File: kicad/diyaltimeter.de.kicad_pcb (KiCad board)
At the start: 2 copper layers, 45.7 x 73.7 mm, 8 parts, among them J1 Buttons, J2 Display, J3 links, J4 rechts, J5 I2C_BMP280, J6 I2C_BMP280_2, J7 RTC DS3231

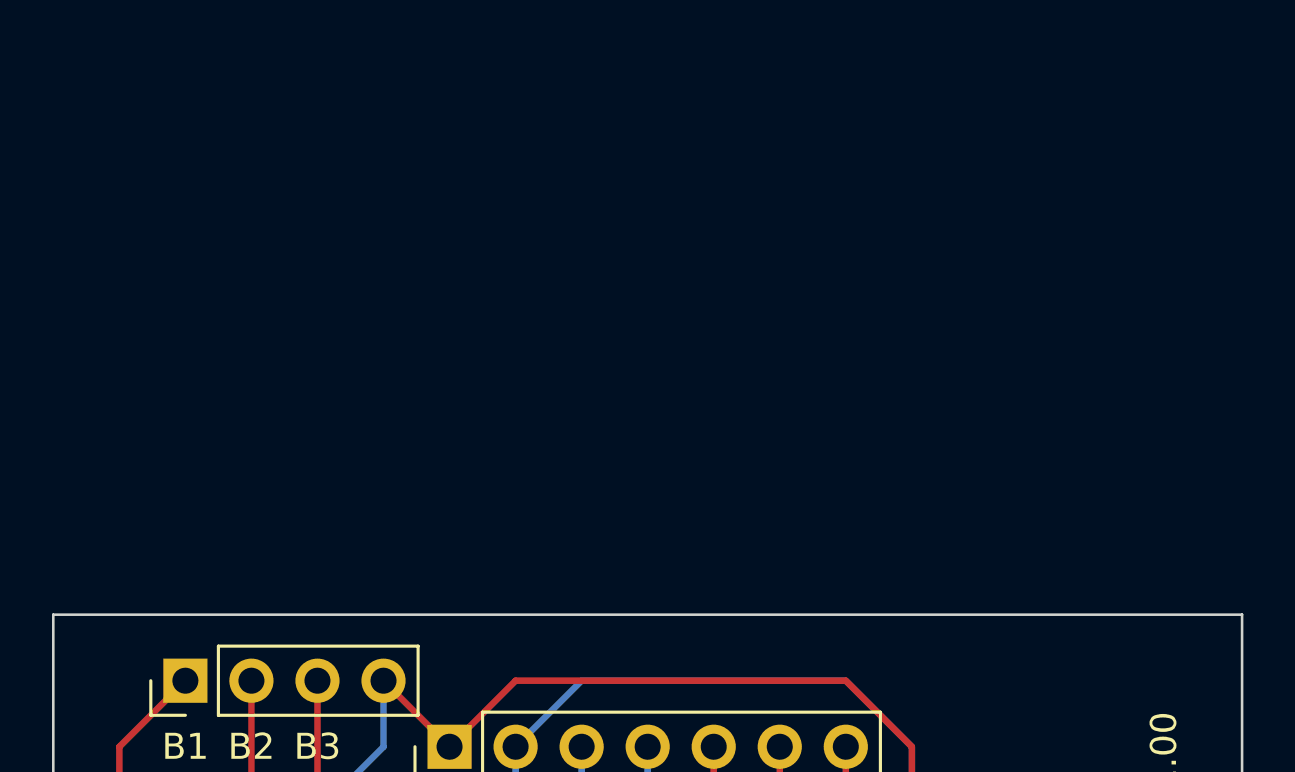
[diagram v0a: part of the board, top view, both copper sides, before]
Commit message: updated pcb
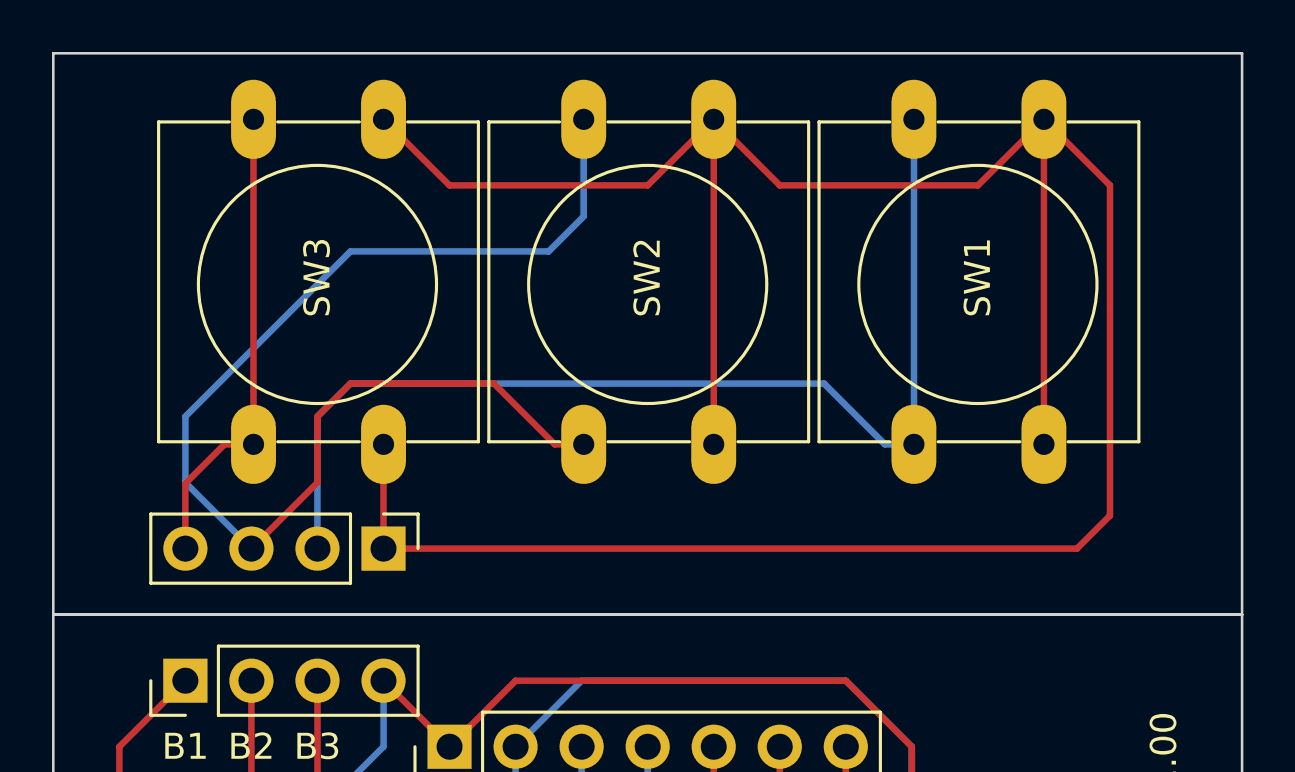
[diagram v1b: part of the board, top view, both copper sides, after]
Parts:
- added J8: Conn_01x04_Male, Connector_PinHeader_2.54mm:PinHeader_1x04_P2.54mm_Vertical, F.Cu at (78.7, 104.1)
- added SW1: SW_Push, Button_Switch_THT:SW_PUSH-12mm, F.Cu at (104.1, 87.6)
- added SW2: SW_Push, Button_Switch_THT:SW_PUSH-12mm, F.Cu at (91.4, 87.6)
- added SW3: SW_Push, Button_Switch_THT:SW_PUSH-12mm, F.Cu at (78.7, 87.6)
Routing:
- net Net-(J8-Pad1): track 0.00 -> 103.4 mm
- net Net-(J8-Pad3): track 0.00 -> 46.2 mm
- net Net-(J8-Pad2): track 0.00 -> 42.7 mm
- net Net-(J8-Pad4): track 0.00 -> 18.2 mm
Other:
- board size 45.7 x 73.7 mm -> 45.7 x 95.2 mm
- net class Default: trace_width 0.25 -> 0.4
- rule trace_min: 0.2 -> 0.4

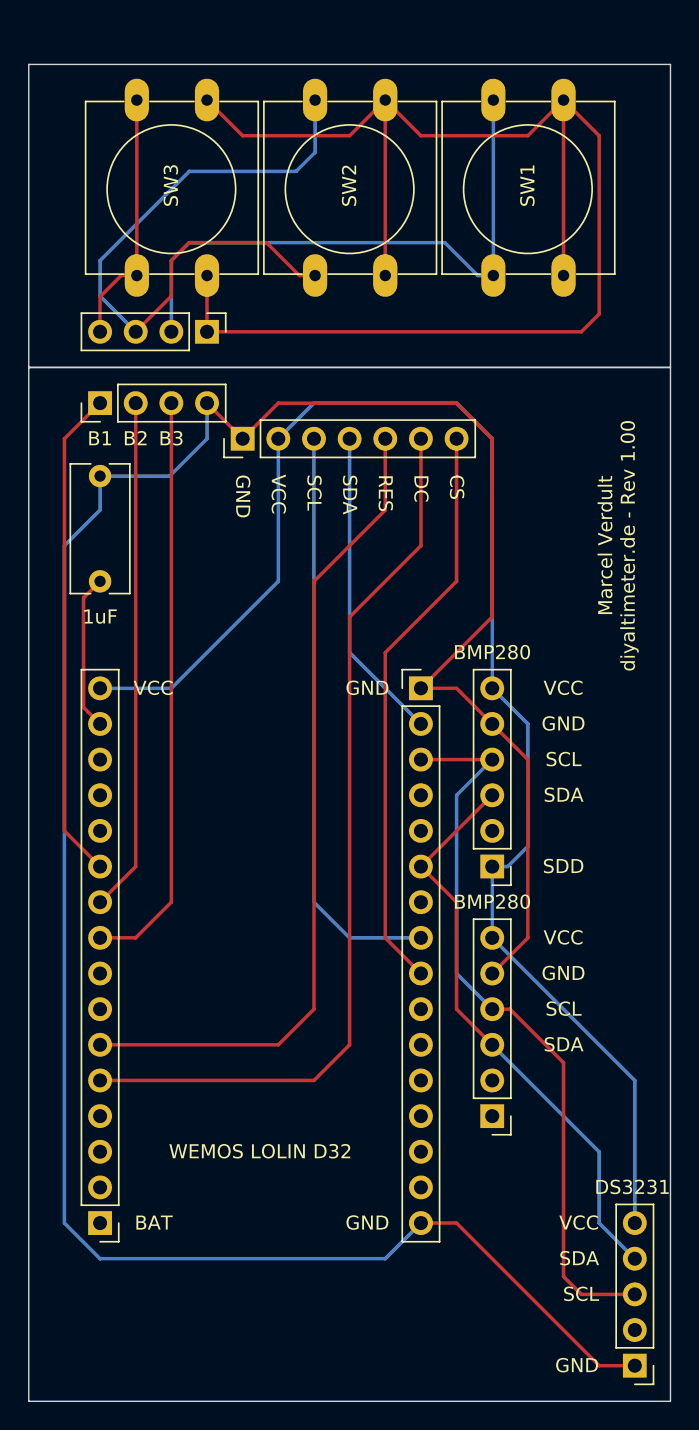
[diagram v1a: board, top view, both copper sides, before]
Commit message: pcb v1.01
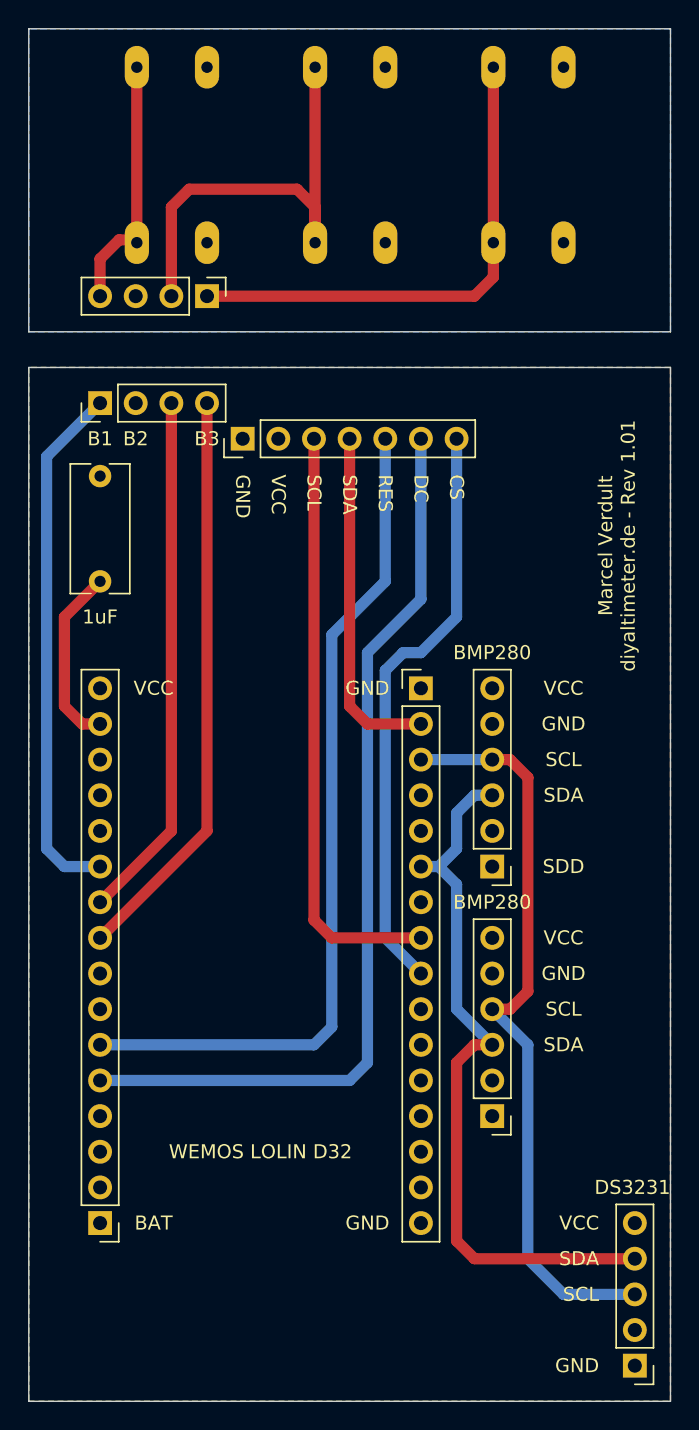
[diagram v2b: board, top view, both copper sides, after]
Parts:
- SW1, SW2, SW3: moved to B.Cu
- moved SW1 10.2 mm to (104.1, 97.8), turned to 90 degrees
- moved SW2 10.2 mm to (91.4, 97.8), turned to 90 degrees
- moved SW3 10.2 mm to (78.7, 97.8), turned to 90 degrees
- moved J8 2.54 mm to (78.7, 101.6)
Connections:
- J1 pad 2: 33 -> GND
- J1 pad 3: 25 -> 33
- J1 pad 4: GND -> 25
- SW1 pad 1: Net-(J8-Pad1) -> Net-(J8-Pad3)
- SW1 pad 2: Net-(J8-Pad2) -> Net-(J8-Pad1)
- SW2 pad 1: Net-(J8-Pad1) -> Net-(J8-Pad3)
- SW2 pad 2: Net-(J8-Pad3) -> Net-(J8-Pad2)
- SW3 pad 1: Net-(J8-Pad1) -> Net-(J8-Pad3)
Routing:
- net GND: track 181.9 -> 0.00 mm
- net +3V3: track 106.2 -> 0.00 mm, vias 0 -> 1
- net Net-(J8-Pad1): track 103.4 -> 36.1 mm
- net Net-(J8-Pad3): track 46.2 -> 0.00 mm
- net I2C_SDA: track 41.4 -> 51.9 mm
- net Net-(J8-Pad2): track 42.7 -> 33.6 mm
- net 32: track 35.1 -> 37.7 mm
- net SDA: track 22.4 -> 24.7 mm
- net RS: track 11.1 -> 13.0 mm
- net DC: track 64.1 -> 65.6 mm
- net RES: track 59.0 -> 60.5 mm
- net I2C_SCL: track 52.5 -> 54.0 mm
- net 33: track 36.6 -> 37.7 mm
- net SCL: track 41.7 -> 42.4 mm
- net CS: track 41.3 -> 42.0 mm
- added copper zone on B.Cu, net +3V3
- added copper zone on F.Cu, net GND
- added copper zone on B.Cu, net Net-(J8-Pad3)
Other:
- board size 45.7 x 95.2 mm -> 45.7 x 97.8 mm
- net class Default: trace_width 0.4 -> 0.8
- rule trace_min: 0.4 -> 0.8
- board text added: "Marcel Verdult diyaltimeter.de - Rev 1.01"
- board text removed: "Marcel Verdult diyaltimeter.de - Rev 1.00"
